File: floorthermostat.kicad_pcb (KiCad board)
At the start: 2 copper layers, 29 parts, among them J1 Temp sensor socket 3 pin, J2 spi7segdisp, J3 Conn_01x06_Socket, J5 Programmin connector, Q1 BC549, SW1 Reset pushbutton, SW2 Enable pushbutton, U1 ESP32-WROOM-32, U2 GOLD 240V 3A SSR, U3 BD33FC0FP, U4 DS18B20

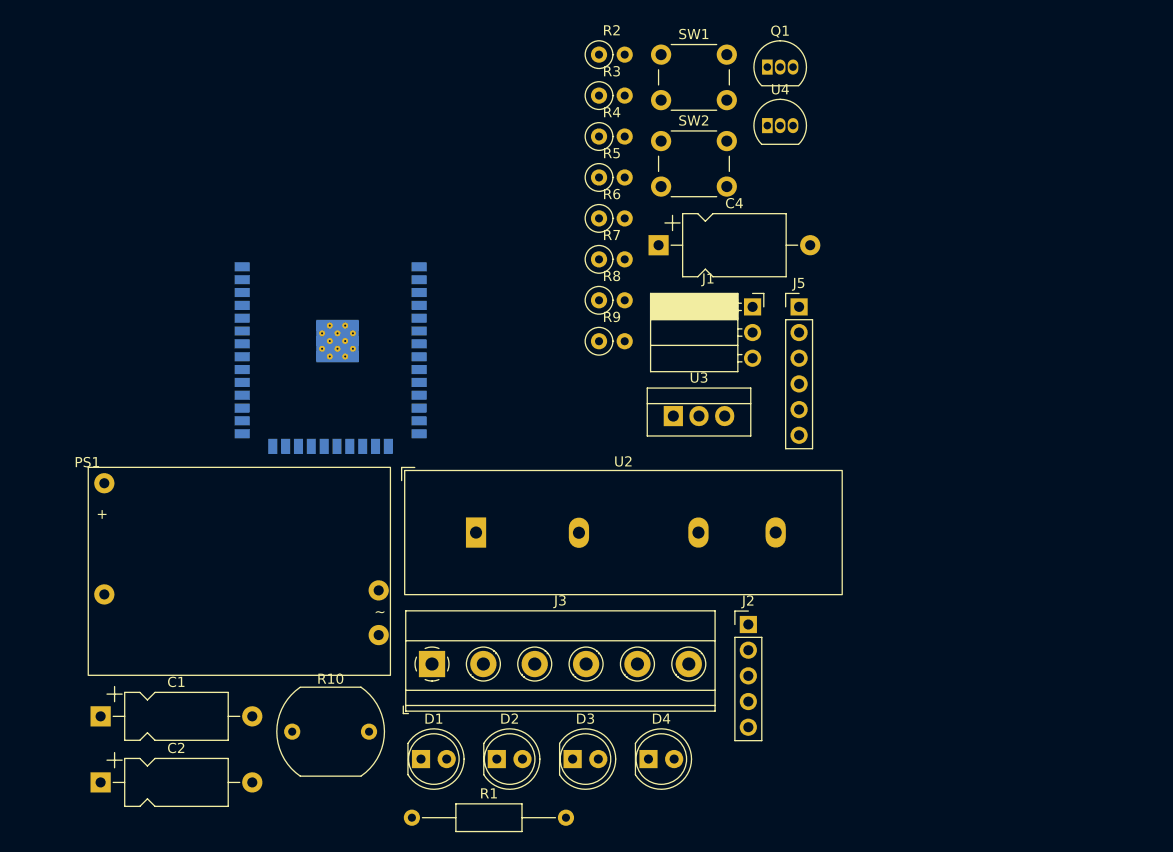
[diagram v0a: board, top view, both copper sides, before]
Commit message: Started designing the pcb.
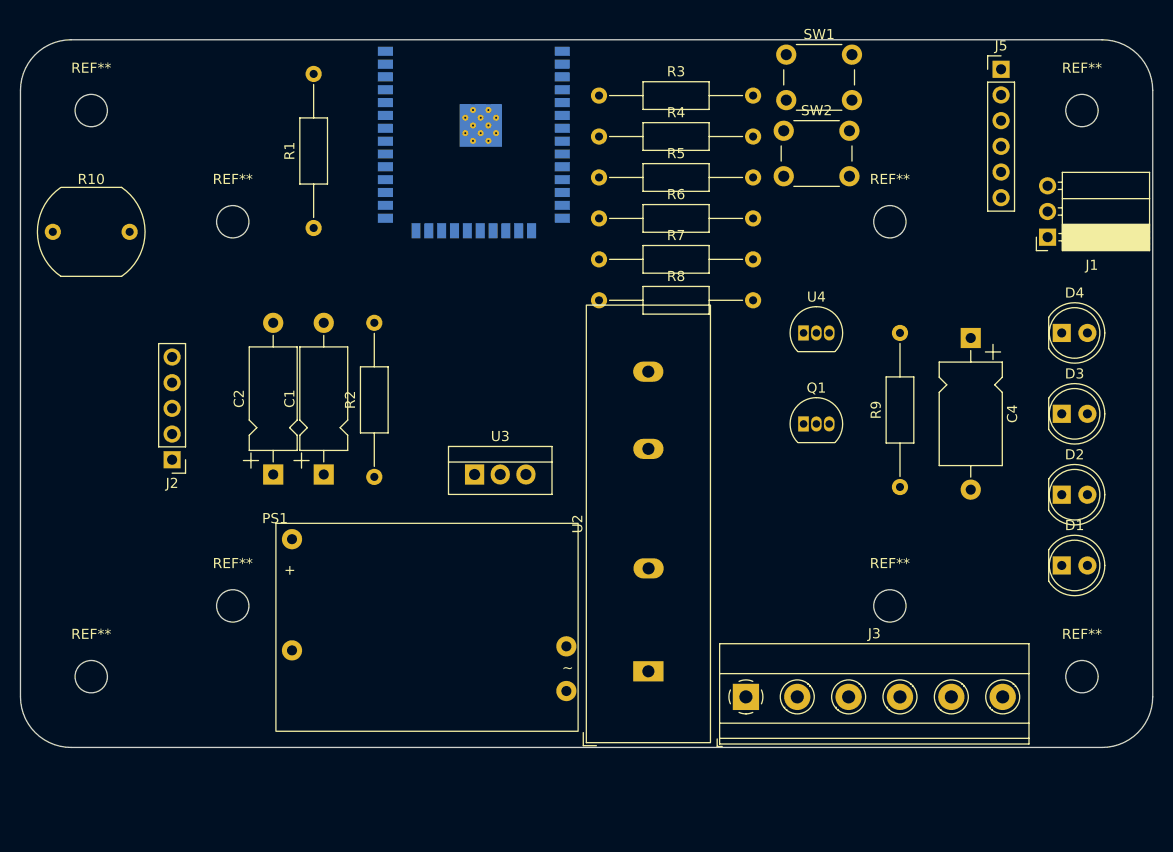
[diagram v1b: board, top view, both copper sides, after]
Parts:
- added REF**: MountingHole_3.2mm_M3, MountingHole:MountingHole_3.2mm_M3, F.Cu at (131.0, 92.0)
- added REF**: MountingHole_3.2mm_M3, MountingHole:MountingHole_3.2mm_M3, F.Cu at (33.0, 92.0)
- added REF**: MountingHole_3.2mm_M3, MountingHole:MountingHole_3.2mm_M3, F.Cu at (47.0, 47.0)
- added REF**: MountingHole_3.2mm_M3, MountingHole:MountingHole_3.2mm_M3, F.Cu at (112.0, 85.0)
- added REF**: MountingHole_3.2mm_M3, MountingHole:MountingHole_3.2mm_M3, F.Cu at (33.0, 36.0)
- added REF**: MountingHole_3.2mm_M3, MountingHole:MountingHole_3.2mm_M3, F.Cu at (112.0, 47.0)
- added REF**: MountingHole_3.2mm_M3, MountingHole:MountingHole_3.2mm_M3, F.Cu at (47.0, 85.0)
- added REF**: MountingHole_3.2mm_M3, MountingHole:MountingHole_3.2mm_M3, F.Cu at (131.0, 36.0)
- R2, R3, R4, R5, R6, R7, R8, R9: footprint Resistor_THT:R_Axial_DIN0207_L6.3mm_D2.5mm_P2.54mm_Vertical -> Resistor_THT:R_Axial_DIN0207_L6.3mm_D2.5mm_P15.24mm_Horizontal
- moved D1 66.2 mm to (129.0, 81.0)
- moved D2 61.7 mm to (129.0, 74.0)
- moved J2 59.3 mm to (41.0, 70.5), turned to 180 degrees
- moved D3 59.2 mm to (129.0, 66.0)
- moved R1 59.1 mm to (55.0, 47.6), turned to 90 degrees
- moved D4 58.7 mm to (129.0, 58.0)
- moved R10 54.8 mm to (29.2, 48.0)
- moved R2 47.3 mm to (61.0, 72.2), turned to 90 degrees
- moved Q1 35.5 mm to (103.5, 67.0)
- moved C2 34.9 mm to (51.0, 72.0), turned to 90 degrees
- moved R9 33.1 mm to (113.0, 73.2), turned to 90 degrees
- moved C1 32.5 mm to (56.0, 72.0), turned to 90 degrees
- moved C4 32.2 mm to (120.0, 58.5), turned to -90 degrees
- moved J3 31.2 mm to (97.8, 94.0)
- moved J5 30.8 mm to (123.0, 31.9)
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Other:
- board outline added: 112 x 70 mm
